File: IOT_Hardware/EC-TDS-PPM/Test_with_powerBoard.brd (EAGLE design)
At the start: 107.2 x 98.4 mm, 188 parts, among them IC1 TL084D, IC2 TL082P, IC3 TL084P, IC4 LINEAR_MC33269ST-3.3T3, IC5 TL082D, IC6 LM2596S, IC7 7805TV, J4 DCJ0202, Q1 NPN, Q2 VSK_N_FET_TO23, Q3 VSK_N_FET_TO23, Q4 VSK_N_FET_TO23, Q5 VSK_N_FET_TO23, Q6 VSK_N_FET_TO23, Q7 32.768, X1 BU-SMA-H

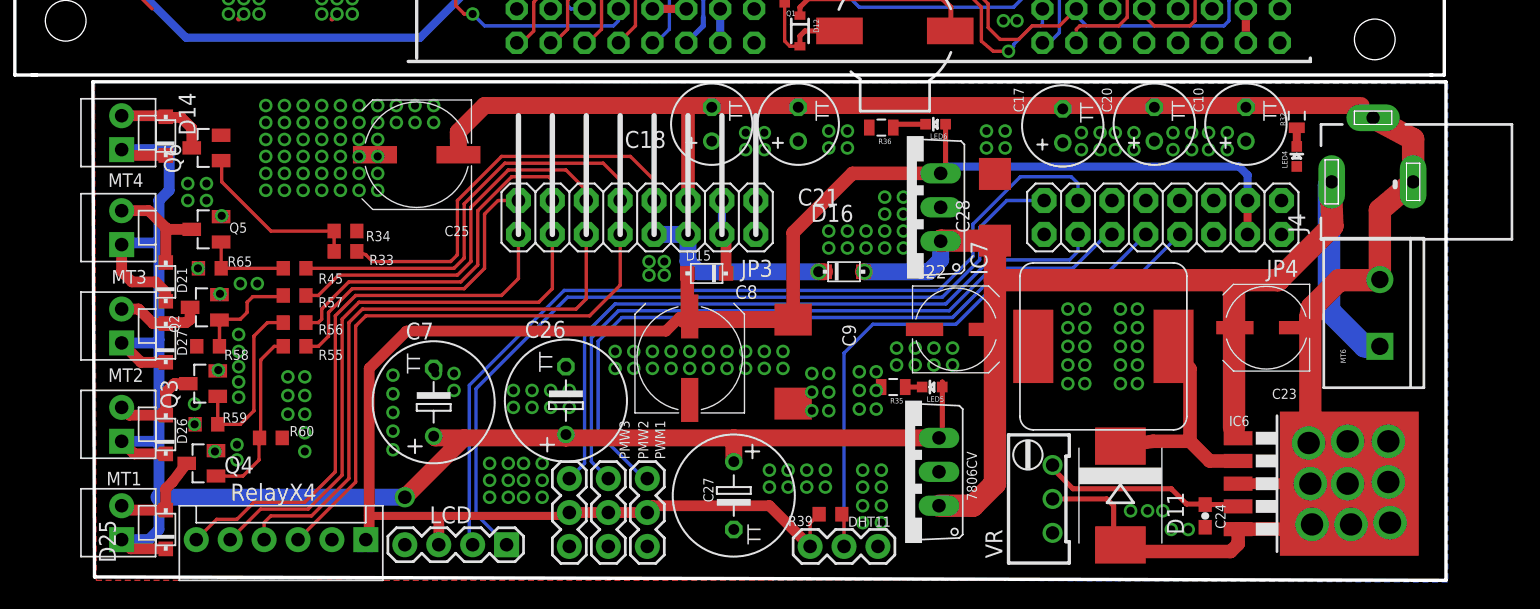
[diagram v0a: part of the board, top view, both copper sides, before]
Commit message: Bang Nguyen Signed-off-by: BangNguyen <ndbn200491@gmail.com>
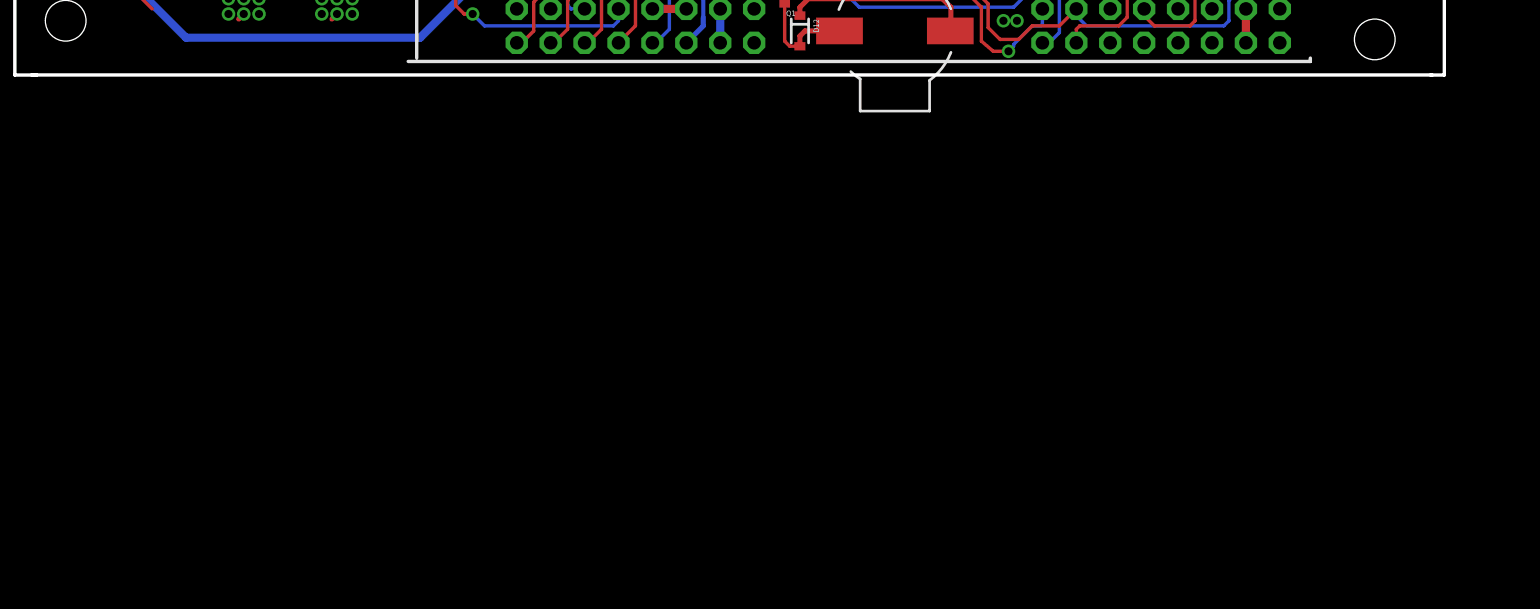
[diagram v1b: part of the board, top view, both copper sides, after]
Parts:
- removed 7806CV: 7806TV, linear:TO220V
- removed C10, C17, C18, C20, C21: 16V 10uF, rcl:TT2D6
- removed C22: 16V 10uF, rcl:UD-6,3X7,7_NICHICON
- removed C23: 35v 100uF, rcl:UD-6,3X7,7_NICHICON
- removed C24: 0.1u, Robotech_RCL:SPARKFUN_0603-CAP
- removed C25: 16V 10uF, rcl:UD-8X10_NICHICON
- removed C26, C27, C7: 35v 100uF, rcl:TT5D9
- removed C28: 35v 100uF, rcl:SMC_C
- removed C8: 35v 100uF, rcl:UD-8X10_NICHICON
- removed C9: 16V 10uF, rcl:SMC_D
- removed D11: MBRS330T3, Robotech Diode of Chung:SMC
- removed D14, D15, D16, D21, D25, D26, D27: PMEG2010AEH, Enleka_Diode:SOT123F
- removed DHT11, PMW2, PMW3, PWM1: (no value), SparkFun-Connectors:1X03
- removed IC6: LM2596S, national-semiconductor:TO263-5
- removed IC7: 7805TV, linear:TO220V
- removed J4: DCJ0202, con-jack:DCJ0202
- removed JP15: (no value), SparkFun-Connectors:MOLEX-1X6
- removed JP3, JP4: (no value), SparkFun-Connectors:2X8
- removed LCD: (no value), SparkFun-Connectors:1X04
- removed LED4, LED5, LED6: (no value), Robotech RLC of Chung:SPARKFUN_LED-0603
- removed MT1: MT1, SparkFun-Connectors:MOLEX-1X2
- removed MT2, MT3, MT4, MT5: (no value), SparkFun-Connectors:MOLEX-1X2
- removed MT6: (no value), SparkFun-Connectors:SCREWTERMINAL-5MM-2
- removed Q2, Q3, Q4, Q5, Q6: VSK_N_FET_TO23, transistor-fet:SOT23
- removed R32, R35, R36: (no value), Robotech_RCL:SPARKFUN_0805
- removed R33, R45, R55, R56, R57: 1K, resistor:R0603
- removed R34, R39, R58, R59, R60, R65: 10k, resistor:R0603
- removed U$9: BIG_INDUCTOR, Big_inductor:12X12
- removed VR: R_TRIM64W_BANG, rtrim:RTRIM64W_BANG
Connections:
- removed net +5V1: C8.+, C9.+, D15.A, DHT11.3, IC7.3, JP15.1, JP4.3, JP4.4, LCD.3, LED6.A, PMW2.2, PMW3.2, PWM1.2, R39.1
- removed net +6V: 7806CV.3, C26.+, C27.+, C7.+, D14.C, D21.C, D25.C, D26.C, D27.C, LED5.A, MT1.1, MT2.1, MT3.1, MT4.1, MT5.1
- removed net +VCC: 7806CV.1, C22.+, C23.+, C28.+, D16.A, IC6.1, IC7.1, J4.1, MT6.1
- removed net -VCC: C10.-, C17.-, C18.-, C20.-, C21.-, C23.-, C25.-, D11.A, IC6.3, IC6.5, IC6.6, J4.2, J4.3, JP3.5, MT6.2, R32.2, VR.2
- removed net CTR2: JP15.3, JP3.10
- removed net CTR3: JP15.4, JP3.12
- removed net CTR4: JP15.5, JP3.14
- removed net CTR5: JP15.6, JP3.16
- removed net CTR_MT1: JP3.15, R55.2
- removed net CTR_MT2: JP3.13, R56.2
- removed net CTR_MT3: JP3.11, R57.2
- removed net CTR_MT4: JP3.9, R45.2
- removed net CTR_MT5: JP3.7, R33.2
- removed net DHT1: DHT11.2, JP4.8, R39.2
- removed net GND2: 7806CV.2, C10.+, C17.+, C18.+, C20.+, C21.+, C22.-, C24.2, C25.+, C26.-, C27.-, C28.-, C7.-, C8.-, C9.-, DHT11.1, IC7.2, JP15.2, JP3.1, JP3.2, JP4.1, JP4.2, LCD.4, LED4.A, PMW2.3, PMW3.3, PWM1.3, Q2.2, Q3.2, Q4.2, Q5.2, Q6.2, R34.2, R35.2, R36.2, R58.2, R59.2, R60.2, R65.2, U$9.P$1, VR.1
- removed net N: D16.C, JP3.6, JP3.8
- removed net N$34: LED4.C, R32.1
- removed net N$35: D26.A, MT2.2, Q3.3
- removed net N$56: D27.A, MT3.2, Q2.3
- removed net N$57: D25.A, MT1.2, Q4.3
- removed net N$58: Q2.1, R57.1, R58.1
- removed net N$59: Q3.1, R56.1, R59.1
- removed net N$60: D21.A, MT4.2, Q5.3
- removed net N$61: Q4.1, R55.1, R60.1
- removed net N$65: Q5.1, R45.1, R65.1
- removed net N$66: D14.A, MT5.2, Q6.3
- removed net N$67: Q6.1, R33.1, R34.1
- removed net N$70: D15.C, JP3.3, JP3.4
- removed net N$73: C24.1, IC6.4, VR.3
- removed net N$74: LED5.C, R35.1
- removed net N$75: LED6.C, R36.1
- removed net OUT1: D11.C, IC6.2, U$9.P$2
- removed net PWM6: JP4.10, PWM1.1
- removed net PWM7: JP4.12, PMW2.1
- removed net PWM8: JP4.14, PMW3.1
- removed net SCL2: JP4.15, LCD.1
- removed net SDA2: JP4.13, LCD.2
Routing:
- net -VCC: track 222.6 -> 0.00 mm, vias 9 -> 0
- net +5V1: track 143.2 -> 0.00 mm
- net +6V: track 141.9 -> 0.00 mm, vias 1 -> 0
- net +VCC: track 98.3 -> 0.00 mm, vias 1 -> 0
- net SDA2: track 67.0 -> 0.00 mm
- net SCL2: track 62.4 -> 0.00 mm
- net PWM6: track 56.3 -> 0.00 mm
- net PWM7: track 53.3 -> 0.00 mm
- net PWM8: track 52.1 -> 0.00 mm
- net DHT1: track 45.8 -> 0.00 mm
- net CTR3: track 44.0 -> 0.00 mm
- net CTR4: track 42.8 -> 0.00 mm
- net CTR2: track 42.7 -> 0.00 mm
- net CTR5: track 42.4 -> 0.00 mm
- net CTR_MT4: track 31.5 -> 0.00 mm
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- removed copper zone on layer 16, net +5V1
- removed copper zone on layer 1, net GND2
- removed copper zone on layer 16, net GND2
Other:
- board size 107.2 x 98.4 mm -> 107.1 x 60.6 mm
- board text removed: "MT1"
- board text removed: "MT2"
- board text removed: "MT3"
- board text removed: "MT4"
- board text removed: "RelayX4"
